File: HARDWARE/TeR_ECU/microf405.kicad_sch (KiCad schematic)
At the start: 24 parts, among them J1 FTSH-105-01-L-DV-K-TR, SW1 RST, U6 STM32F405VGTx, X2 ASE-xxxMHz

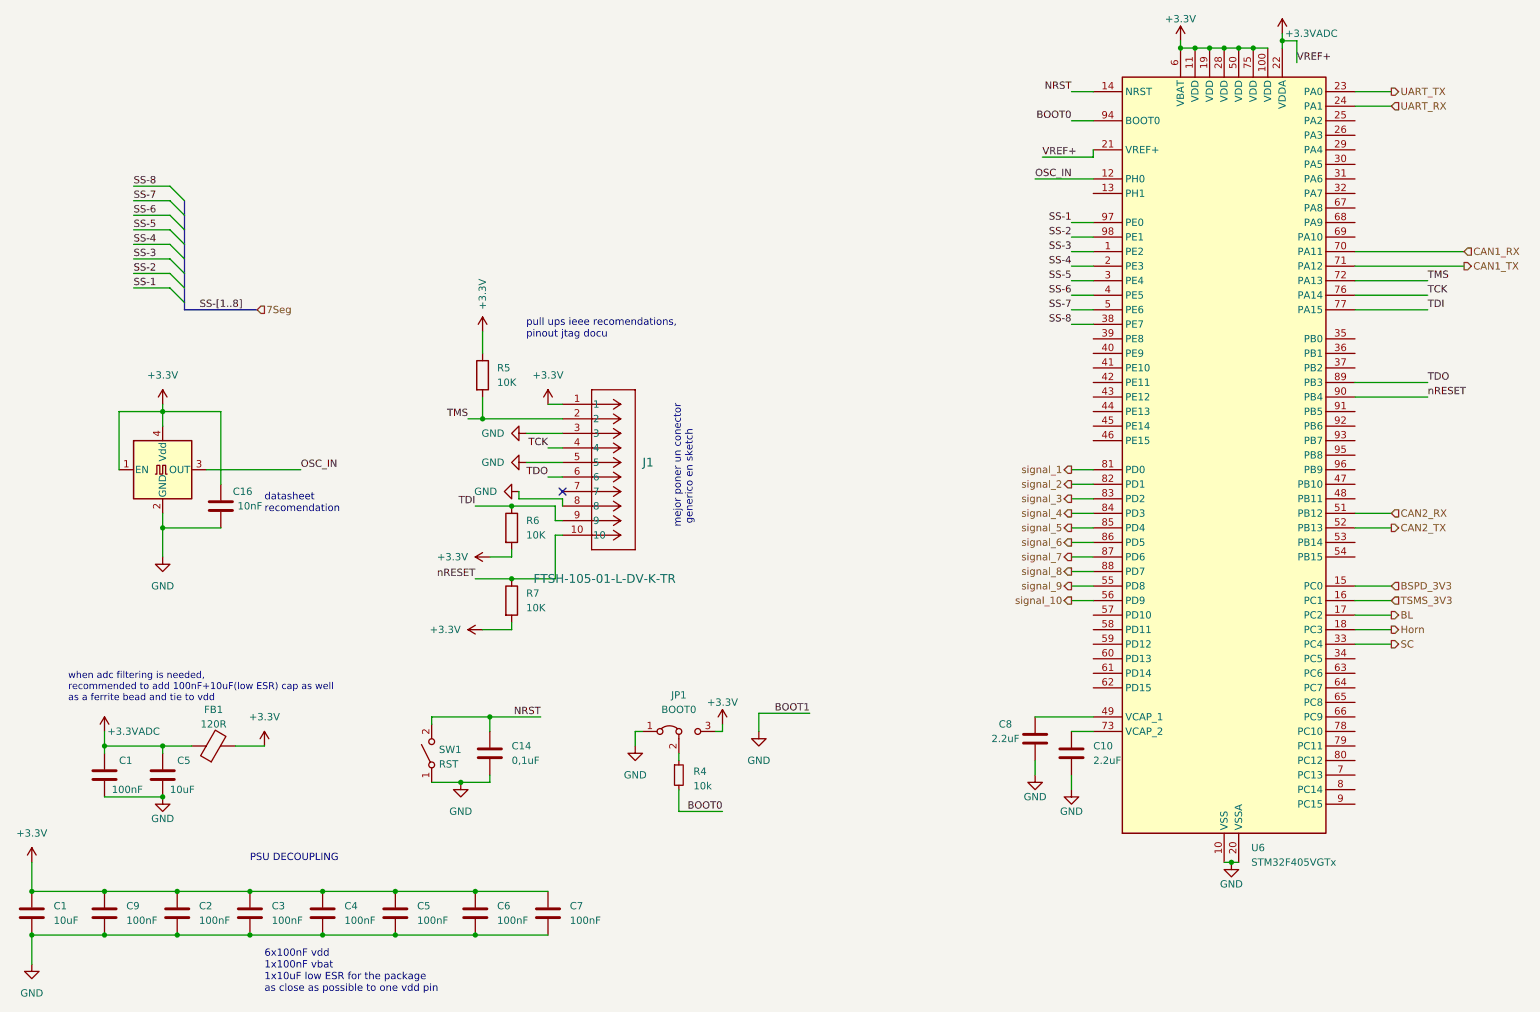
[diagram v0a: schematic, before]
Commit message: ic comments
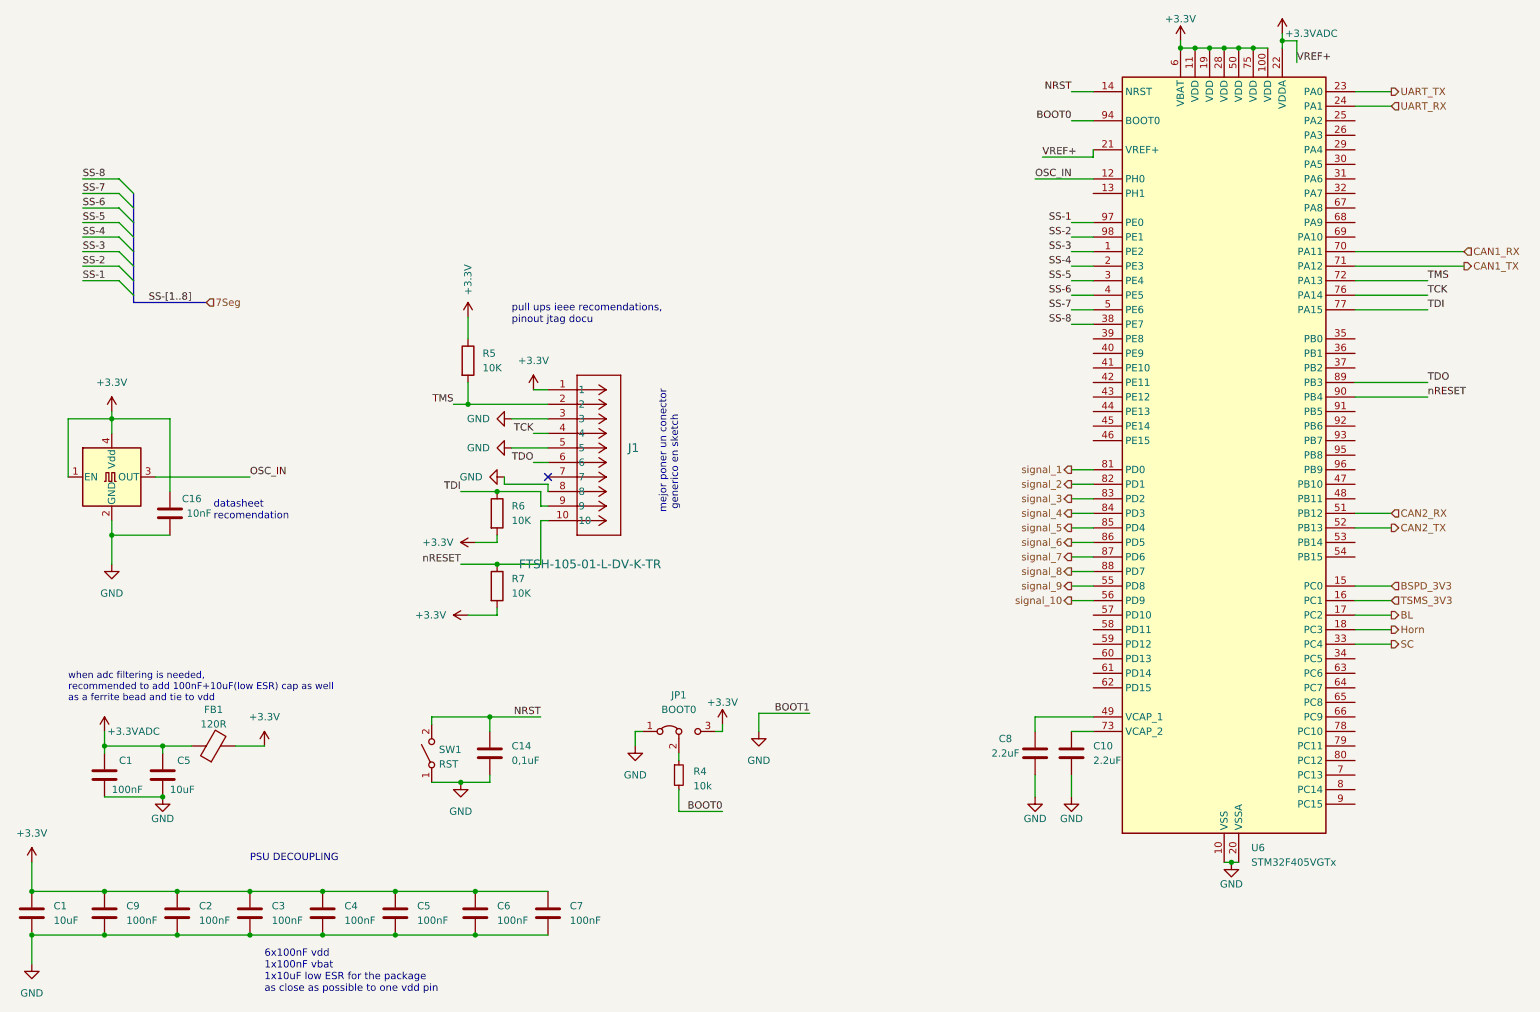
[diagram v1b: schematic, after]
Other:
- moved on the sheet: C16, C8, J1, R5, R6, R7
